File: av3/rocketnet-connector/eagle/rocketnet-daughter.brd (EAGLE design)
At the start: 18.8 x 8.8 mm, 11 parts

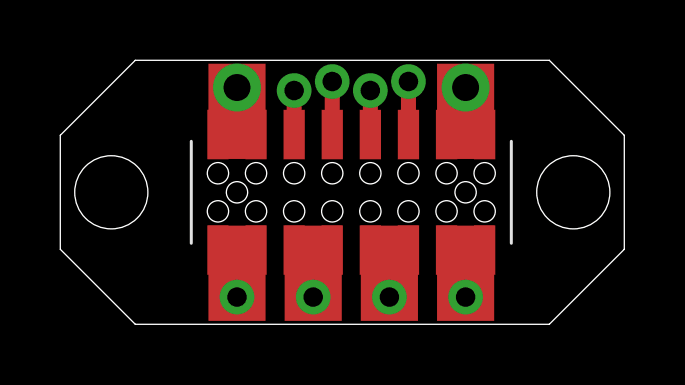
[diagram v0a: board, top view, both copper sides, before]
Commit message: Updated rocketnet connectors and boards to match new rocketnet stackup.
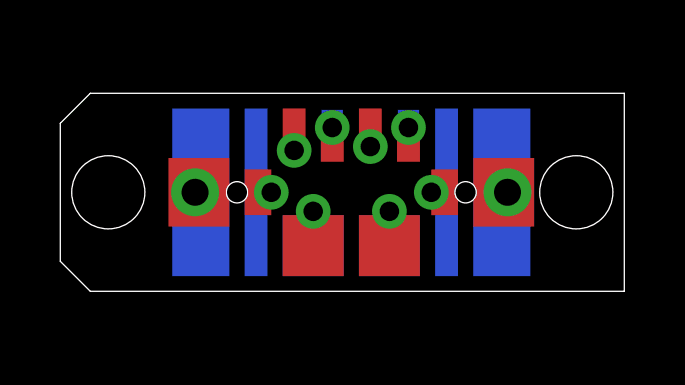
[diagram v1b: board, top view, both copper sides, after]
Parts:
- removed E$3, E$5, E$6, E$7: (no value), rocketnet-connector:26AWG-WIRE
- added E$12, E$13, E$14, E$15: (no value), rocketnet-connector:26AWG-WIRE
- E$2: device rocketnet-connector:HARWIN-M50-31508 -> rocketnet-connector:HARWIN-M50-31508-NO-HOLES
- moved E$1 3.76 mm to (-5.21, 0.00)
- moved E$4 3.76 mm to (5.21, 0.00)
- moved E$8 2.00 mm to (-1.91, 1.40)
- moved E$10 1.87 mm to (0.64, 1.52)
- moved E$11 1.53 mm to (1.91, 2.16)
- moved E$9 1.53 mm to (-0.64, 2.16)
- flipped E$2 to the bottom
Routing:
- net S$4: track 1.95 -> 0.00 mm
- net S$5: track 1.81 -> 0.00 mm
- net S$1: track 1.79 -> 0.00 mm
- net S$2: track 1.49 -> 0.00 mm
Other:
- board size 18.8 x 8.8 mm -> 18.8 x 6.6 mm
- board text added: "TOP VIEW (M50 on bottom of board)"
- board text removed: "TOP VIEW (M50 on top of board)"
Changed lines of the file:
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@@
 <board>
 <plain>
-<wire x1="9.1" y1="-1.9" x2="9.1" y2="1.9" width="0.02" layer="20"/>
-<wire x1="6.6" y1="-4.4" x2="-7.2" y2="-4.4" width="0.02" layer="20"/>
-<wire x1="-9.7" y1="-1.9" x2="-9.7" y2="1.9" width="0.02" layer="20"/>
-<text x="-10.194" y="8.116" size="0.762" layer="48">TOP VIEW (M50 on top of board)</text>
-<text x="3.2" y="4.8" size="0.762" layer="48">B-</text>
-<text x="-0.3" y="4.8" size="0.762" layer="48" rot="R90">AUX2</text>
-<text x="-1.6" y="4.8" size="0.762" layer="48" rot="R90">AUX1</text>
-<text x="-2.2" y="-5.3" size="0.762" layer="48">RX-</text>
-<text x="-4.8" y="-5.3" size="0.762" layer="48">RX+</text>
-<text x="2.9" y="-5.3" size="0.762" layer="48">TX-</text>
-<text x="0.4" y="-5.3" size="0.762" layer="48">TX+</text>
-<text x="-4.2" y="4.8" size="0.762" layer="48">B+</text>
-<hole x="7.4" y="0" drill="2.4384"/>
-<hole x="-8" y="0" drill="2.4384"/>
-<text x="0.9" y="4.8" size="0.762" layer="48" rot="R90">AUX3</text>
-<text x="2.2" y="4.8" size="0.762" layer="48" rot="R90">AUX4</text>
-<rectangle x1="-2.2225" y1="-4.28625" x2="-0.3175" y2="-1.11125" layer="1"/>
-<rectangle x1="-4.7625" y1="-4.28625" x2="-2.8575" y2="-1.11125" layer="1"/>
-<rectangle x1="0.3175" y1="-4.28625" x2="2.2225" y2="-1.11125" layer="1"/>
-<rectangle x1="2.8575" y1="-4.28625" x2="4.7625" y2="-1.11125" layer="1"/>
-<rectangle x1="2.8575" y1="1.11125" x2="4.7625" y2="4.28625" layer="1"/>
-<rectangle x1="-4.7625" y1="1.11125" x2="-2.8575" y2="4.28625" layer="1"/>
-<wire x1="6.6" y1="4.4" x2="-7.2" y2="4.4" width="0.02" layer="20"/>
-<wire x1="-9.7" y1="1.9" x2="-7.2" y2="4.4" width="0.02" layer="20"/>
-<wire x1="-7.2" y1="-4.4" x2="-9.7" y2="-1.9" width="0.02" layer="20"/>
-<wire x1="9.1" y1="-1.9" x2="6.6" y2="-4.4" width="0.02" layer="20"/>
-<wire x1="6.6" y1="4.4" x2="9.1" y2="1.9" width="0.02" layer="20"/>
-<wire x1="-9.15" y1="-2" x2="-6.85" y2="-2" width="0.01" layer="51"/>
-<wire x1="-6.85" y1="-2" x2="-5.7" y2="0" width="0.01" layer="51"/>
-<wire x1="-5.7" y1="0" x2="-6.85" y2="2" width="0.01" layer="51"/>
-<wire x1="-6.85" y1="2" x2="-9.15" y2="2" width="0.01" layer="51"/>
-<wire x1="-9.15" y1="2" x2="-10.3" y2="0" width="0.01" layer="51"/>
-<wire x1="-10.3" y1="0" x2="-9.15" y2="-2" width="0.01" layer="51"/>
-<wire x1="6.25" y1="-2" x2="8.55" y2="-2" width="0.01" layer="51"/>
-<wire x1="8.55" y1="-2" x2="9.7" y2="0" width="0.01" layer="51"/>
-<wire x1="9.7" y1="0" x2="8.55" y2="2" width="0.01" layer="51"/>
-<wire x1="8.55" y1="2" x2="6.25" y2="2" width="0.01" layer="51"/>
-<wire x1="6.25" y1="2" x2="5.1" y2="0" width="0.01" layer="51"/>
-<wire x1="5.1" y1="0" x2="6.25" y2="-2" width="0.01" layer="51"/>
-<text x="10.05" y="-2.3" size="0.762" layer="48">#2-56 nylock
+<wire x1="9.1" y1="-3.3" x2="9.1" y2="3.3" width="0.02" layer="20"/>
+<wire x1="9.1" y1="-3.3" x2="-8.7" y2="-3.3" width="0.02" layer="20"/>
+<wire x1="-8.7" y1="-3.3" x2="-9.7" y2="-2.3" width="0.02" layer="20"/>
+<wire x1="-9.7" y1="-2.3" x2="-9.7" y2="2.3" width="0.02" layer="20"/>
+<wire x1="-9.7" y1="2.3" x2="-8.7" y2="3.3" width="0.02" layer="20"/>
+<text x="-10.194" y="8.116" size="0.762" layer="48">TOP VIEW (M50 on bottom of board)</text>
+<text x="4.3" y="4.1" size="0.762" layer="48">B-</text>
+<text x="-0.4" y="3.8" size="0.762" layer="48" rot="R90">AUX2</text>
+<text x="-1.7" y="3.8" size="0.762" layer="48" rot="R90">AUX1</text>
+<text x="-1.9" y="-4.4" size="0.762" layer="48">RX-</text>
+<text x="-2.8" y="-5.4" size="0.762" layer="48" rot="R90">RX+</text>
+<text x="3.7" y="-5.4" size="0.762" layer="48" rot="R90">TX-</text>
+<text x="0.6" y="-4.4" size="0.762" layer="48">TX+</text>
+<text x="-5.5" y="4" size="0.762" layer="48">B+</text>
+<hole x="7.5" y="0" drill="2.4384"/>
+<hole x="-8.1" y="0" drill="2.4384"/>
+<text x="0.8" y="3.8" size="0.762" layer="48" rot="R90">AUX3</text>
+<text x="2.1" y="3.8" size="0.762" layer="48" rot="R90">AUX4</text>
+<wire x1="9.1" y1="3.3" x2="-8.7" y2="3.3" width="0.02" layer="20"/>
+<text x="9.85" y="-1.2" size="0.762" layer="48">#2-56 nylock
 (5/32" OD)</text>
+<circle x="-1.905" y="-0.635" radius="0.356503125" width="0.0254" layer="52"/>
+<circle x="-4.445" y="0.635" radius="0.356503125" width="0.0254" layer="52"/>
+<circle x="-4.445" y="-0.635" radius="0.356503125" width="0.0254" layer="52"/>
+<circle x="-3.175" y="-0.635" radius="0.356503125" width="0.0254" layer="52"/>
+<circle x="-3.175" y="0.635" radius="0.356503125" width="0.0254" layer="52"/>
+<circle x="-1.905" y="0.635" radius="0.356503125" width="0.0254" layer="52"/>
+<circle x="-0.635" y="0.635" radius="0.356503125" width="0.0254" layer="52"/>
+<circle x="-0.635" y="-0.635" radius="0.356503125" width="0.0254" layer="52"/>
+<circle x="0.635" y="0.635" radius="0.356503125" width="0.0254" layer="52"/>
+<circle x="0.635" y="-0.635" radius="0.356503125" width="0.0254" layer="52"/>
+<circle x="1.905" y="0.635" radius="0.356503125" width="0.0254" layer="52"/>
+<circle x="1.905" y="-0.635" radius="0.356503125" width="0.0254" layer="52"/>
+<circle x="3.175" y="0.635" radius="0.356503125" width="0.0254" layer="52"/>
+<circle x="3.175" y="-0.635" radius="0.356503125" width="0.0254" layer="52"/>
+<circle x="4.445" y="0.635" radius="0.356503125" width="0.0254" layer="52"/>
+<circle x="4.445" y="-0.635" radius="0.356503125" width="0.0254" layer="52"/>
+<rectangle x1="4.064" y1="-2.794" x2="5.969" y2="2.794" layer="16"/>
+<rectangle x1="-5.969" y1="-2.794" x2="-4.064" y2="2.794" layer="16"/>
+<rectangle x1="-2.286" y1="-2.794" x2="-0.254" y2="-0.762" layer="16"/>
+<rectangle x1="2.794" y1="-2.794" x2="3.556" y2="2.794" layer="16"/>
+<rectangle x1="-3.556" y1="-2.794" x2="-2.794" y2="2.794" layer="16"/>
+<rectangle x1="-2.286" y1="-2.794" x2="-0.254" y2="-0.762" layer="1"/>
+<rectangle x1="0.254" y1="-2.794" x2="2.286" y2="-0.762" layer="16"/>
+<rectangle x1="0.254" y1="-2.794" x2="2.286" y2="-0.762" layer="1"/>
+<rectangle x1="-2.286" y1="1.397" x2="-1.524" y2="2.794" layer="1"/>
+<rectangle x1="-1.016" y1="1.016" x2="-0.254" y2="2.159" layer="1"/>
+<rectangle x1="0.254" y1="1.524" x2="1.016" y2="2.794" layer="1"/>
+<rectangle x1="1.524" y1="1.016" x2="2.286" y2="2.159" layer="1"/>
+<rectangle x1="-6.096" y1="-1.143" x2="-4.064" y2="1.143" layer="1"/>
+<rectangle x1="4.064" y1="-1.143" x2="6.096" y2="1.143" layer="1"/>
+<rectangle x1="2.667" y1="-0.762" x2="3.556" y2="0.762" layer="1"/>
+<rectangle x1="-3.556" y1="-0.762" x2="-2.667" y2="0.762" layer="1"/>
 </plain>
 <attributes>
@@
 </autorouter>
 <elements>
-<element name="E$2" library="rocketnet-connector" package="HARWIN-M50-31508" value="" x="0" y="0"/>
-<element name="E$1" library="rocketnet-connector" package="22AWG-WIRE" value="" x="-3.81" y="3.4925"/>
-<element name="E$3" library="rocketnet-connector" package="26AWG-WIRE" value="" x="-3.81" y="-3.4925"/>
-<element name="E$4" library="rocketnet-connector" package="22AWG-WIRE" value="" x="3.81" y="3.4925"/>
-<element name="E$5" library="rocketnet-connector" package="26AWG-WIRE" value="" x="-1.27" y="-3.4925"/>
-<element name="E$6" library="rocketnet-connector" package="26AWG-WIRE" value="" x="1.27" y="-3.4925"/>
-<element name="E$7" library="rocketnet-connector" package="26AWG-WIRE" value="" x="3.81" y="-3.4925"/>
-<element name="E$8" library="rocketnet-connector" package="26AWG-WIRE" value="" x="-1.905" y="3.3925"/>
-<element name="E$9" library="rocketnet-connector" package="26AWG-WIRE" value="" x="-0.635" y="3.6925"/>
-<element name="E$10" library="rocketnet-connector" package="26AWG-WIRE" value="" x="0.635" y="3.3925"/>
-<element name="E$11" library="rocketnet-connector" package="26AWG-WIRE" value="" x="1.905" y="3.6925"/>
+<element name="E$2" library="rocketnet-connector" package="HARWIN-M50-31508-NO-HOLES" value="" x="0" y="0" rot="MR0"/>
+<element name="E$1" library="rocketnet-connector" package="22AWG-WIRE" value="" x="-5.207" y="0"/>
+<element name="E$4" library="rocketnet-connector" package="22AWG-WIRE" value="" x="5.207" y="0"/>
+<element name="E$8" library="rocketnet-connector" package="26AWG-WIRE" value="" x="-1.905" y="1.397"/>
+<element name="E$9" library="rocketnet-connector" package="26AWG-WIRE" value="" x="-0.635" y="2.159"/>
+<element name="E$10" library="rocketnet-connector" package="26AWG-WIRE" value="" x="0.635" y="1.524"/>
+<element name="E$11" library="rocketnet-connector" package="26AWG-WIRE" value="" x="1.905" y="2.159"/>
+<element name="E$12" library="rocketnet-connector" package="26AWG-WIRE" value="" x="-2.667" y="0"/>
+<element name="E$13" library="rocketnet-connector" package="26AWG-WIRE" value="" x="-1.27" y="-0.635"/>
+<element name="E$14" library="rocketnet-connector" package="26AWG-WIRE" value="" x="1.27" y="-0.635"/>
+<element name="E$15" library="rocketnet-connector" package="26AWG-WIRE" value="" x="2.667" y="0"/>
 </elements>
 <signals>
@@
 <signal name="S$1">
 <contactref element="E$11" pad="P$1"/>
-<wire x1="1.905" y1="3.6925" x2="1.905" y2="1.905" width="0.5" layer="1"/>
 </signal>
 <signal name="S$2">
 <contactref element="E$10" pad="P$1"/>
-<wire x1="0.635" y1="3.3925" x2="0.635" y2="1.905" width="0.5" layer="1"/>
 </signal>
 <signal name="S$4">
 <contactref element="E$9" pad="P$1"/>
-<wire x1="-0.635" y1="3.6925" x2="-0.635" y2="1.74625" width="0.5" layer="1"/>
 </signal>
 <signal name="S$5">
 <contactref element="E$8" pad="P$1"/>
-<wire x1="-1.905" y1="3.3925" x2="-1.905" y2="1.5875" width="0.5" layer="1"/>
 </signal>
 </signals>
